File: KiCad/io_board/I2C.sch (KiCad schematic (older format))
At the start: 6 parts, among them J5 DS1307, J6 BME280, U17 PCA9564D

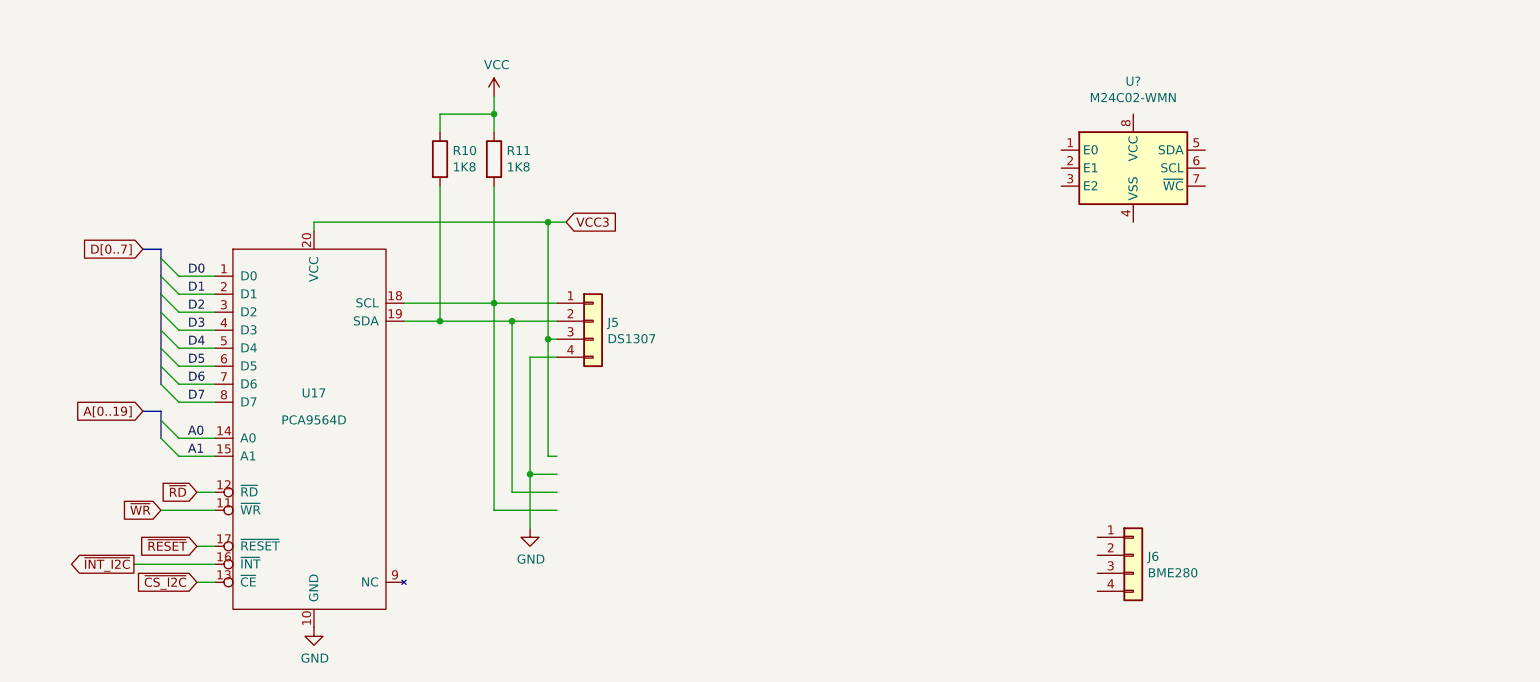
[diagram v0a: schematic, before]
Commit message: Worked on I/O board.
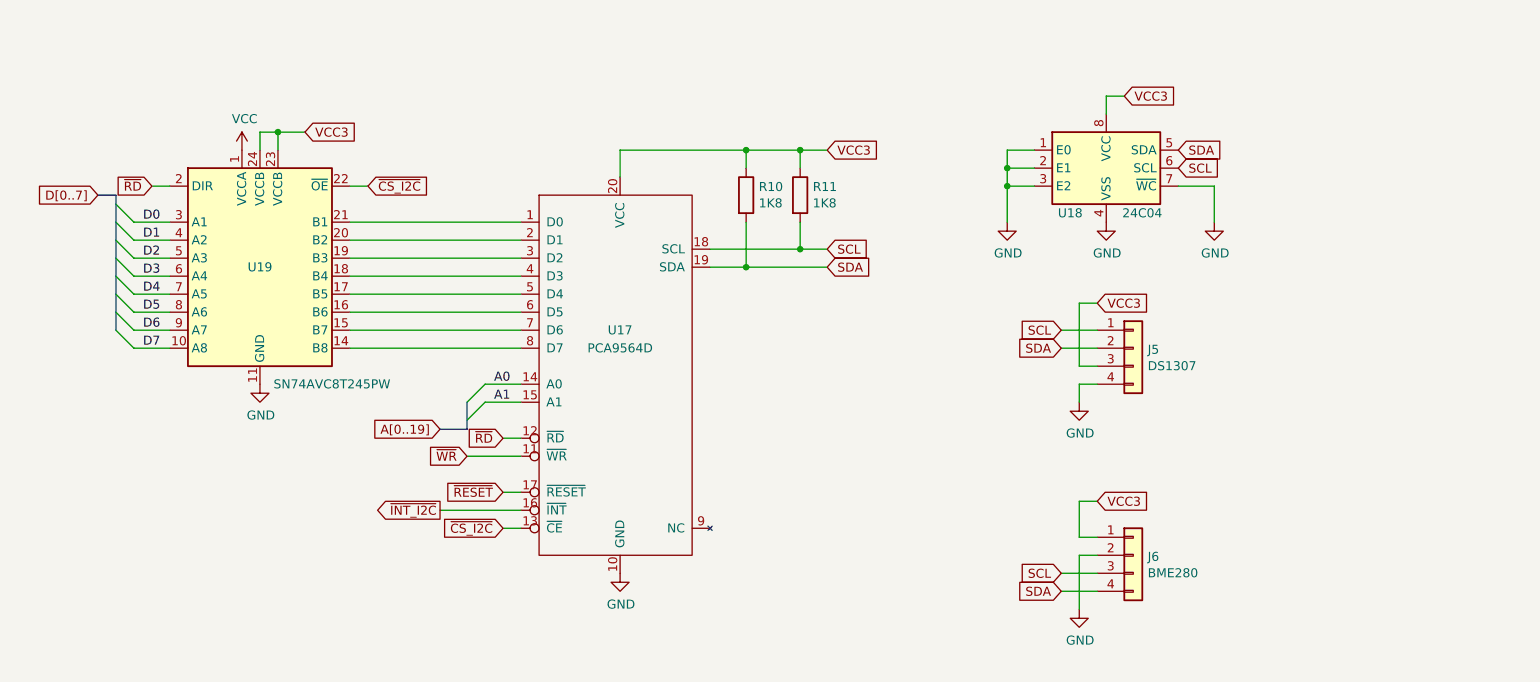
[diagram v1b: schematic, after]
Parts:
- added U19: SN74AVC8T245PW, Package_SO:TSSOP-24_4.4x7.8mm_P0.65mm, symbol Logic_LevelTranslator:SN74AVC8T245PW
- J5, J6: footprint (none) -> Connector_PinHeader_2.54mm:PinHeader_1x04_P2.54mm_Vertical
- R10, R11: footprint (none) -> Resistor_THT:R_Axial_DIN0207_L6.3mm_D2.5mm_P2.54mm_Vertical
- U17: footprint (none) -> Package_SO:SOIC-20W_7.5x12.8mm_P1.27mm
- U18: renamed from U?; value M24C02-WMN -> 24C04
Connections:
- net labels added: SCL, SDA
- wire segments 41 -> 65
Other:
- moved on the sheet: J5, R10, R11, U18

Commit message: Continued work on I/O board.
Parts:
- R10, R11: footprint Resistor_THT:R_Axial_DIN0207_L6.3mm_D2.5mm_P2.54mm_Vertical -> Resistor_SMD:R_1206_3216Metric
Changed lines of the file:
@@
 F 0 "R10" H 5270 2146 50  0000 L CNN
 F 1 "1K8" H 5270 2055 50  0000 L CNN
-F 2 "Resistor_THT:R_Axial_DIN0207_L6.3mm_D2.5mm_P2.54mm_Vertical" V 5130 2100 50  0001 C CNN
+F 2 "Resistor_SMD:R_1206_3216Metric" V 5130 2100 50  0001 C CNN
 F 3 "~" H 5200 2100 50  0001 C CNN
 	1    5200 2100
@@
 F 0 "R11" H 5570 2146 50  0000 L CNN
 F 1 "1K8" H 5570 2055 50  0000 L CNN
-F 2 "Resistor_THT:R_Axial_DIN0207_L6.3mm_D2.5mm_P2.54mm_Vertical" V 5430 2100 50  0001 C CNN
+F 2 "Resistor_SMD:R_1206_3216Metric" V 5430 2100 50  0001 C CNN
 F 3 "~" H 5500 2100 50  0001 C CNN
 	1    5500 2100

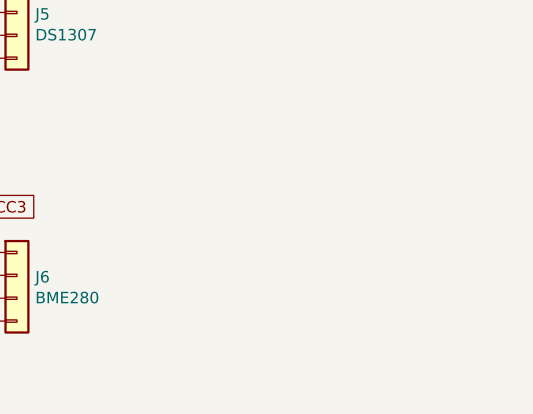
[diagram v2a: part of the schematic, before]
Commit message: Updated I/O board
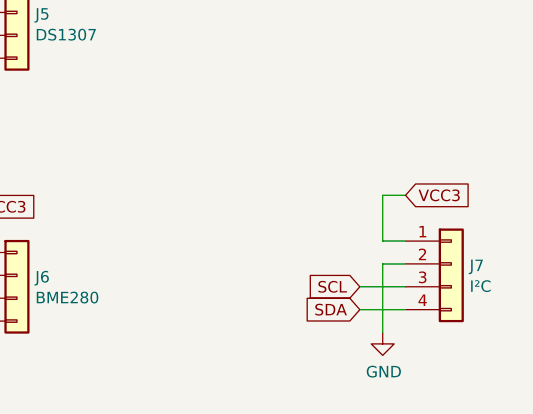
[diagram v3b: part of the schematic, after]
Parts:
- added J7: I²C, Connector_PinHeader_2.54mm:PinHeader_1x04_P2.54mm_Vertical, symbol Connector_Generic:Conn_01x04
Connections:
- net GND: now also J7.2 (Pin_2)
- net SCL: now also J7.3 (Pin_3)
- net SDA: now also J7.4 (Pin_4)
- net VCC3: now also J7.1 (Pin_1)
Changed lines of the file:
@@
 	1    0    0    -1
 $EndComp
+$Comp
+L Connector_Generic:Conn_01x04 J7
+U 1 1 5FDA3AF8
+P 9250 4050
+F 0 "J7" H 9330 4042 50  0000 L CNN
+F 1 "I²C" H 9330 3951 50  0000 L CNN
+F 2 "Connector_PinHeader_2.54mm:PinHeader_1x04_P2.54mm_Vertical" H 9250 4050 50  0001 C CNN
+F 3 "~" H 9250 4050 50  0001 C CNN
+	1    9250 4050
+	1    0    0    -1
+$EndComp
+Wire Wire Line
+	9050 4050 8950 4050
+Wire Wire Line
+	8950 4050 8950 4350
+Wire Wire Line
+	8950 3950 9050 3950
+$Comp
+L power:GND #PWR0113
+U 1 1 5FDA3B01
+P 8950 4350
+F 0 "#PWR0113" H 8950 4100 50  0001 C CNN
+F 1 "GND" H 8955 4177 50  0000 C CNN
+F 2 "" H 8950 4350 50  0001 C CNN
+F 3 "" H 8950 4350 50  0001 C CNN
+	1    8950 4350
+	1    0    0    -1
+$EndComp
+Text GLabel 9050 3750 2    50   Input ~ 0
+VCC3
+Wire Wire Line
+	9050 3750 8950 3750
+Wire Wire Line
+	8950 3750 8950 3950
+Wire Wire Line
+	9050 4150 8850 4150
+Wire Wire Line
+	9050 4250 8850 4250
+Text GLabel 8850 4250 0    50   Input ~ 0
+SDA
+Text GLabel 8850 4150 0    50   Input ~ 0
+SCL
 Wire Bus Line
 	3650 3250 3650 3400

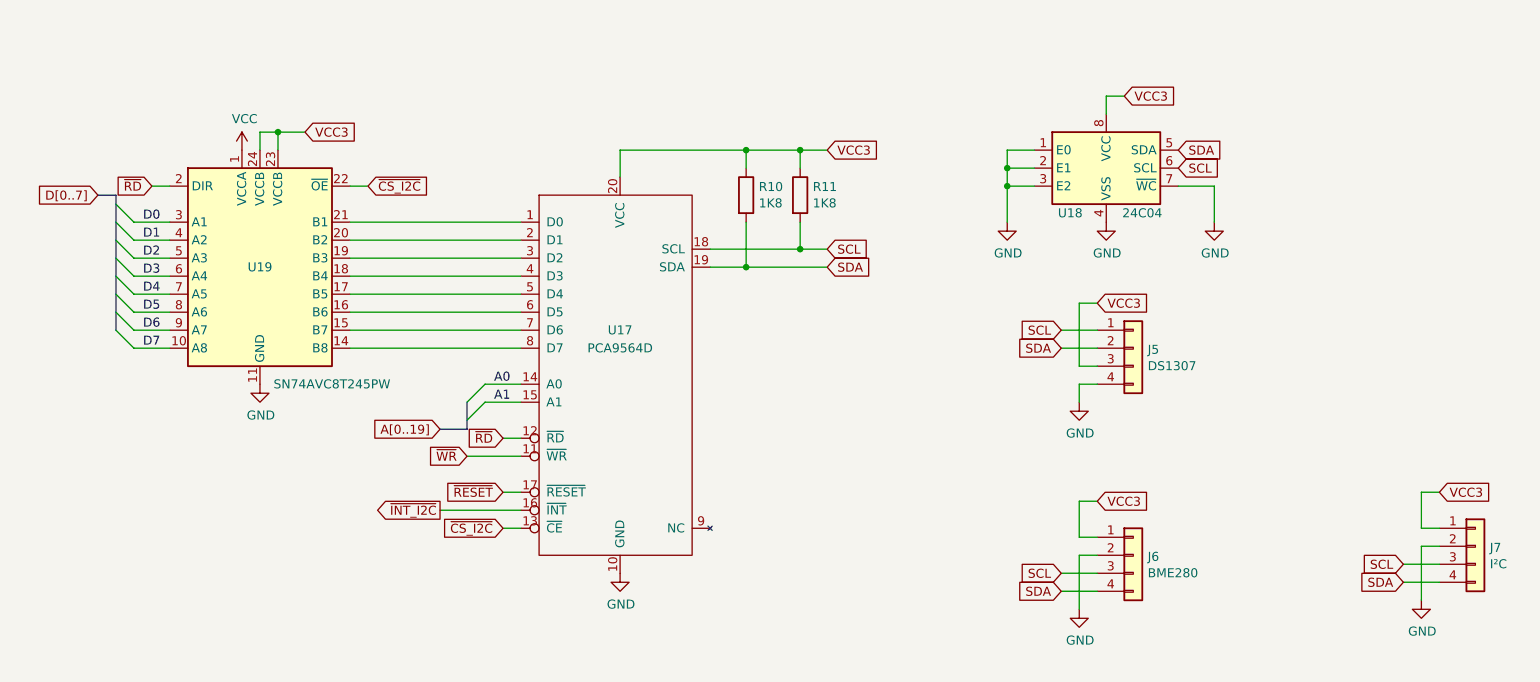
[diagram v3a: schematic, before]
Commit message: Updated I/O board
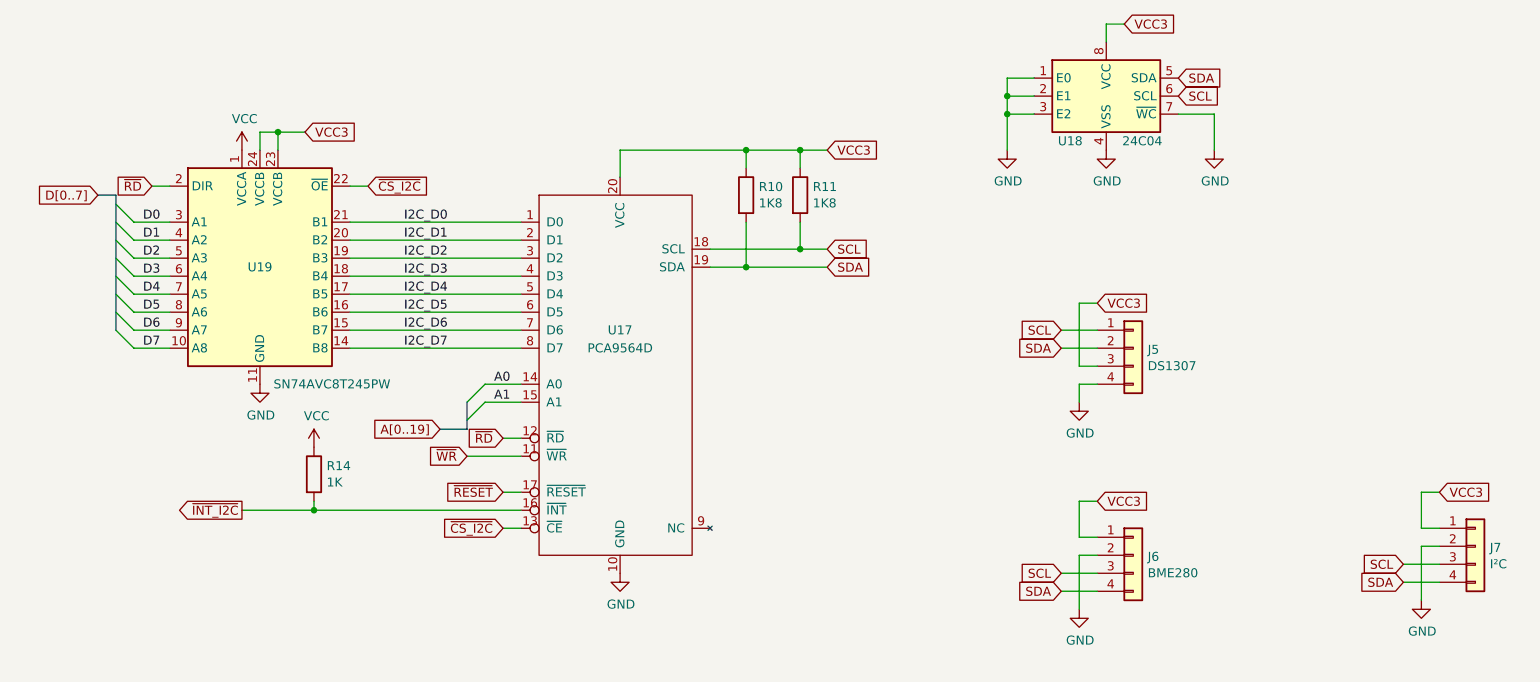
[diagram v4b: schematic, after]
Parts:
- added R14: 1K, Resistor_SMD:R_1206_3216Metric, symbol Device:R
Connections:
- net VCC: now also R14.1
- net ~INT_I2C: now also R14.2
- net I2C_D7: now reaches U17.8 (D7), U19.14 (B8)
- net I2C_D6: now reaches U17.7 (D6), U19.15 (B7)
- net I2C_D5: now reaches U17.6 (D5), U19.16 (B6)
- net I2C_D4: now reaches U17.5 (D4), U19.17 (B5)
- net I2C_D3: now reaches U17.4 (D3), U19.18 (B4)
- net I2C_D2: now reaches U17.3 (D2), U19.19 (B3)
- net I2C_D1: now reaches U17.2 (D1), U19.20 (B2)
- net I2C_D0: now reaches U17.1 (D0), U19.21 (B1)
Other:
- moved on the sheet: U18
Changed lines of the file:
@@
 ~CS_I2C
 Wire Wire Line
-	3950 3850 3500 3850
-Text GLabel 3500 3850 0    50   Output ~ 0
+	3950 3850 2800 3850
+Text GLabel 2400 3850 0    50   Output ~ 0
 ~INT_I2C
 $Comp
@@
 L Memory_EEPROM:M24C02-WMN U18
 U 1 1 5FAFF485
-P 7200 1950
-F 0 "U18" H 7000 1700 50  0000 C CNN
-F 1 "24C04" H 7400 1700 50  0000 C CNN
-F 2 "Package_SO:SOIC-8_3.9x4.9mm_P1.27mm" H 7200 2300 50  0001 C CNN
-F 3 "http://www.st.com/content/ccc/resource/technical/document/datasheet/b0/d8/50/40/5a/85/49/6f/DM00071904.pdf/files/DM00071904.pdf/jcr:content/translations/en.DM00071904.pdf" H 7250 1450 50  0001 C CNN
-	1    7200 1950
+P 7200 1550
+F 0 "U18" H 7000 1300 50  0000 C CNN
+F 1 "24C04" H 7400 1300 50  0000 C CNN
+F 2 "Package_SO:SOIC-8_3.9x4.9mm_P1.27mm" H 7200 1900 50  0001 C CNN
+F 3 "http://www.st.com/content/ccc/resource/technical/document/datasheet/b0/d8/50/40/5a/85/49/6f/DM00071904.pdf/files/DM00071904.pdf/jcr:content/translations/en.DM00071904.pdf" H 7250 1050 50  0001 C CNN
+	1    7200 1550
 	1    0    0    -1
 $EndComp
@@
 L power:GND #PWR0110
 U 1 1 5FB9D832
-P 7200 2250
-F 0 "#PWR0110" H 7200 2000 50  0001 C CNN
-F 1 "GND" H 7205 2077 50  0000 C CNN
-F 2 "" H 7200 2250 50  0001 C CNN
-F 3 "" H 7200 2250 50  0001 C CNN
-	1    7200 2250
-	1    0    0    -1
-$EndComp
-Text GLabel 7300 1550 2    50   Input ~ 0
-VCC3
-Wire Wire Line
-	7300 1550 7200 1550
-Wire Wire Line
-	7200 1550 7200 1650
+P 7200 1850
+F 0 "#PWR0110" H 7200 1600 50  0001 C CNN
+F 1 "GND" H 7205 1677 50  0000 C CNN
+F 2 "" H 7200 1850 50  0001 C CNN
+F 3 "" H 7200 1850 50  0001 C CNN
+	1    7200 1850
+	1    0    0    -1
+$EndComp
+Text GLabel 7300 1150 2    50   Input ~ 0
+VCC3
+Wire Wire Line
+	7300 1150 7200 1150
+Wire Wire Line
+	7200 1150 7200 1250
 Text GLabel 6950 2850 0    50   Input ~ 0
 SCL
@@
 Text GLabel 5650 2500 2    50   Input ~ 0
 SDA
-Text GLabel 7600 1950 2    50   Input ~ 0
-SCL
-Text GLabel 7600 1850 2    50   Input ~ 0
-SDA
-Wire Wire Line
-	7600 2050 7800 2050
+Text GLabel 7600 1550 2    50   Input ~ 0
+SCL
+Text GLabel 7600 1450 2    50   Input ~ 0
+SDA
+Wire Wire Line
+	7600 1650 7800 1650
 $Comp
 L power:GND #PWR0112
 U 1 1 5FBAB9A0
-P 7800 2250
-F 0 "#PWR0112" H 7800 2000 50  0001 C CNN
-F 1 "GND" H 7805 2077 50  0000 C CNN
-F 2 "" H 7800 2250 50  0001 C CNN
-F 3 "" H 7800 2250 50  0001 C CNN
-	1    7800 2250
-	1    0    0    -1
-$EndComp
-Wire Wire Line
-	7800 2250 7800 2050
-Wire Wire Line
-	6800 1850 6650 1850
-Wire Wire Line
-	6650 1850 6650 1950
-Wire Wire Line
-	6800 2050 6650 2050
-Connection ~ 6650 2050
-Wire Wire Line
-	6650 2050 6650 2250
-Wire Wire Line
-	6800 1950 6650 1950
-Connection ~ 6650 1950
-Wire Wire Line
-	6650 1950 6650 2050
+P 7800 1850
+F 0 "#PWR0112" H 7800 1600 50  0001 C CNN
+F 1 "GND" H 7805 1677 50  0000 C CNN
+F 2 "" H 7800 1850 50  0001 C CNN
+F 3 "" H 7800 1850 50  0001 C CNN
+	1    7800 1850
+	1    0    0    -1
+$EndComp
+Wire Wire Line
+	7800 1850 7800 1650
+Wire Wire Line
+	6800 1450 6650 1450
+Wire Wire Line
+	6650 1450 6650 1550
+Wire Wire Line
+	6800 1650 6650 1650
+Connection ~ 6650 1650
+Wire Wire Line
+	6650 1650 6650 1850
+Wire Wire Line
+	6800 1550 6650 1550
+Connection ~ 6650 1550
+Wire Wire Line
+	6650 1550 6650 1650
 $Comp
 L power:GND #PWR045
 U 1 1 5FBBE950
-P 6650 2250
-F 0 "#PWR045" H 6650 2000 50  0001 C CNN
-F 1 "GND" H 6655 2077 50  0000 C CNN
-F 2 "" H 6650 2250 50  0001 C CNN
-F 3 "" H 6650 2250 50  0001 C CNN
-	1    6650 2250
+P 6650 1850
+F 0 "#PWR045" H 6650 1600 50  0001 C CNN
+F 1 "GND" H 6655 1677 50  0000 C CNN
+F 2 "" H 6650 1850 50  0001 C CNN
+F 3 "" H 6650 1850 50  0001 C CNN
+	1    6650 1850
 	1    0    0    -1
 $EndComp
@@
 Text GLabel 8850 4150 0    50   Input ~ 0
 SCL
+Text Label 3300 2250 0    50   ~ 0
+I2C_D0
+Text Label 3300 2350 0    50   ~ 0
+I2C_D1
+Text Label 3300 2450 0    50   ~ 0
+I2C_D2
+Text Label 3300 2550 0    50   ~ 0
+I2C_D3
+Text Label 3300 2650 0    50   ~ 0
+I2C_D4
+Text Label 3300 2750 0    50   ~ 0
+I2C_D5
+Text Label 3300 2850 0    50   ~ 0
+I2C_D6
+Text Label 3300 2950 0    50   ~ 0
+I2C_D7
+$Comp
+L Device:R R14
+U 1 1 5FF0847A
+P 2800 3650
+F 0 "R14" H 2870 3696 50  0000 L CNN
+F 1 "1K" H 2870 3605 50  0000 L CNN
+F 2 "Resistor_SMD:R_1206_3216Metric" V 2730 3650 50  0001 C CNN
+F 3 "~" H 2800 3650 50  0001 C CNN
+	1    2800 3650
+	1    0    0    -1
+$EndComp
+$Comp
+L power:VCC #PWR061
+U 1 1 5FF08EEA
+P 2800 3500
+F 0 "#PWR061" H 2800 3350 50  0001 C CNN
+F 1 "VCC" H 2815 3673 50  0000 C CNN
+F 2 "" H 2800 3500 50  0001 C CNN
+F 3 "" H 2800 3500 50  0001 C CNN
+	1    2800 3500
+	1    0    0    -1
+$EndComp
+Wire Wire Line
+	2800 3800 2800 3850
 Wire Bus Line
 	3650 3250 3650 3400
 Wire Bus Line
 	1700 2100 1700 2850
+Connection ~ 2800 3850
+Wire Wire Line
+	2800 3850 2400 3850
 $EndSCHEMATC
